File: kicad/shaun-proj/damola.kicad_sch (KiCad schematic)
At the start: 34 parts, among them U4 DRV8833PWPR, U6 TPS63020DSJR, U7 DRV8833PWPR, U8 TPS63020DSJR

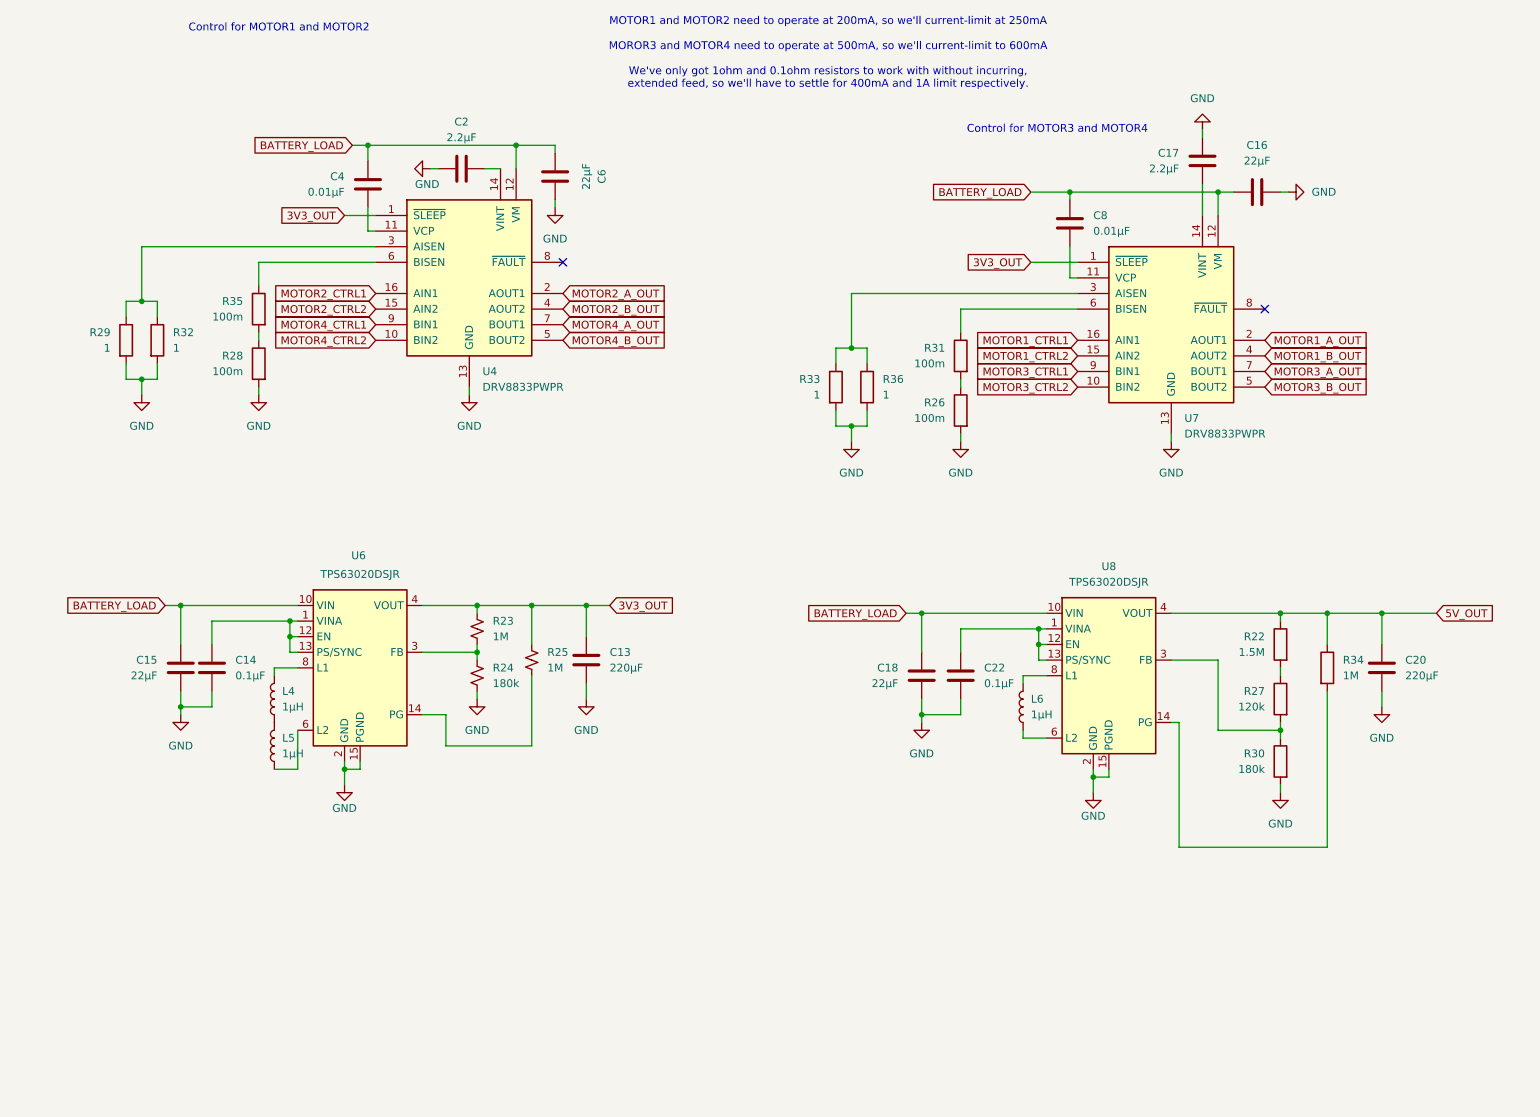
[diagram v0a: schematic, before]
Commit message: schema improvements, cleanup
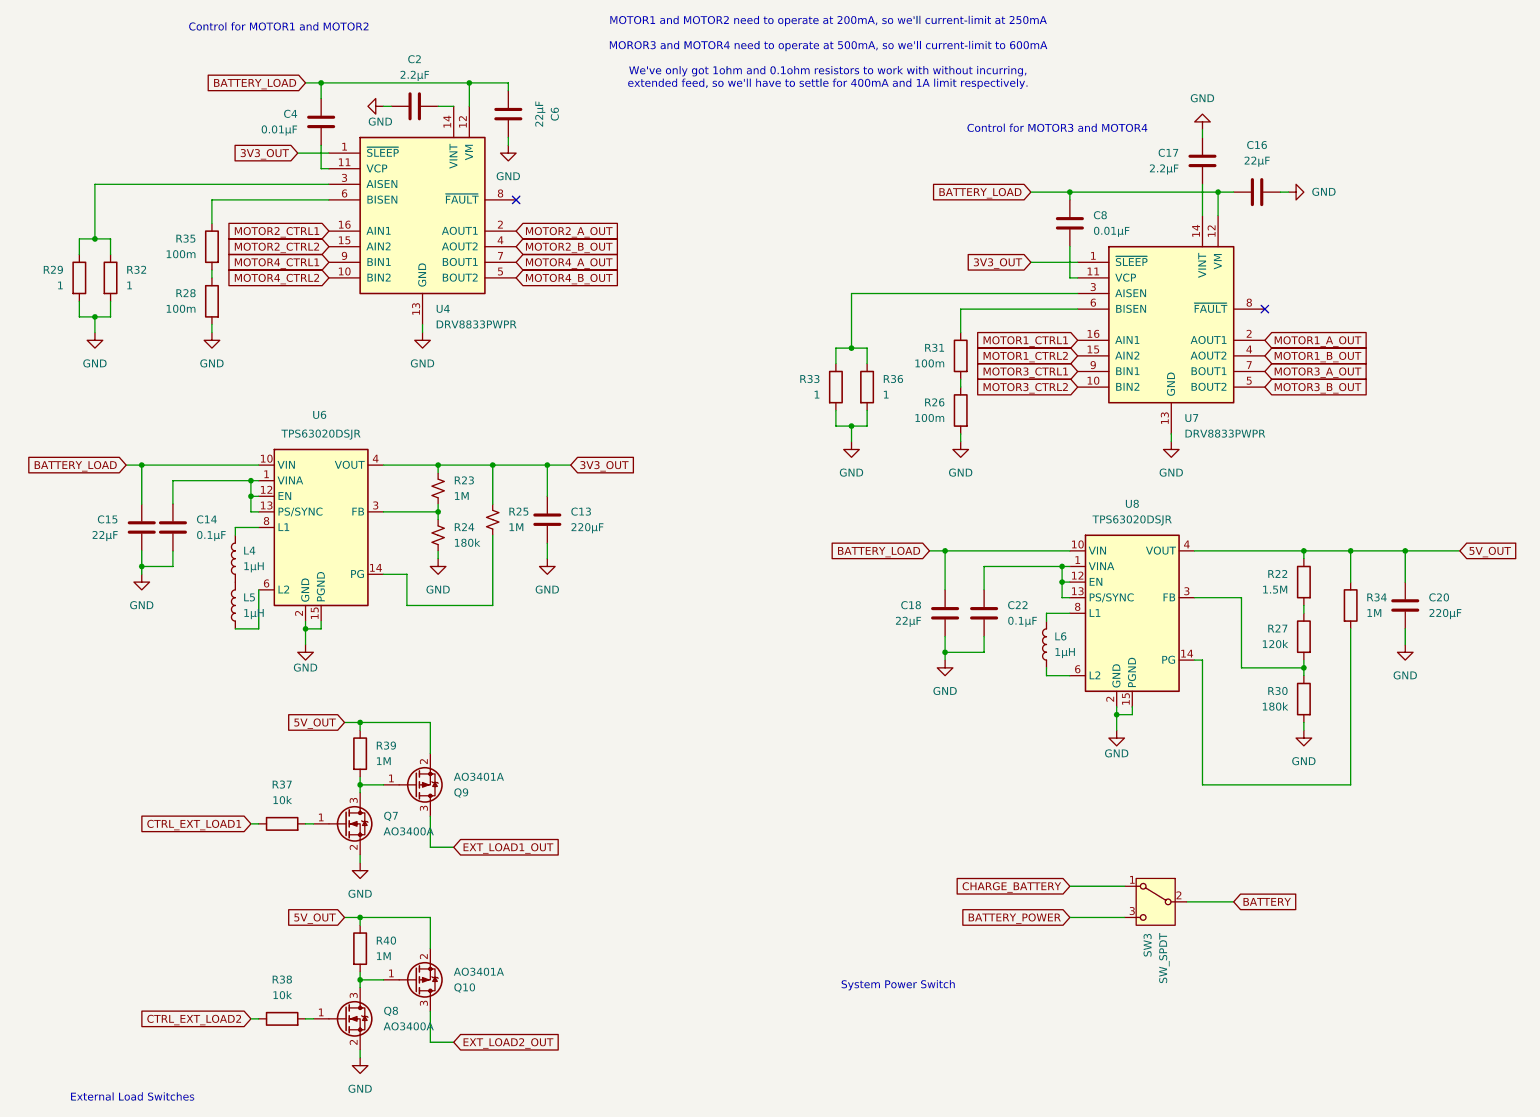
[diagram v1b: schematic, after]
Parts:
- added Q10, Q9: AO3401A, Package_TO_SOT_SMD:SOT-23, symbol Transistor_FET:AO3401A
- added Q7, Q8: AO3400A, Package_TO_SOT_SMD:SOT-23, symbol Transistor_FET:AO3400A
- added R37, R38: 10k, Resistor_SMD:R_0603_1608Metric_Pad0.98x0.95mm_HandSolder, symbol Device:R
- added R39, R40: 1M, Resistor_SMD:R_0603_1608Metric_Pad0.98x0.95mm_HandSolder, symbol Device:R
- added SW3: SW_SPDT, MyLibrary:SS-12D11G3R, symbol Switch:SW_SPDT
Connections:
- net 5V_OUT: now also Q10.2 (S), Q9.2 (S), R39.1, R40.1
- net GND: now also Q7.2 (S), Q8.2 (S)
- new net: Q7.1 (G), R37.2
- new net: Q7.3 (D), Q9.1 (G), R39.2
- new net: Q10.1 (G), Q8.3 (D), R40.2
- new net: Q8.1 (G), R38.2
- new net BATTERY: SW3.2 (B)
- new net BATTERY_POWER: SW3.3 (C)
- new net CHARGE_BATTERY: SW3.1 (A)
- new net CTRL_EXT_LOAD1: R37.1
- new net CTRL_EXT_LOAD2: R38.1
- new net EXT_LOAD1_OUT: Q9.3 (D)
- new net EXT_LOAD2_OUT: Q10.3 (D)
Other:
- note added: "External Load Switches"
- note added: "System Power Switch"
- moved on the sheet: C13, C14, C15, C18, C2, C20, C22, C4, C6, L4, L5, L6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
